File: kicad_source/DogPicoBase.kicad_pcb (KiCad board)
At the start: 2 copper layers, 72 x 53 mm, 52 parts, among them CN1 ARDUINO_ISP, CN2 ARDUINO_MKR, Q1 2N7002, SW1 TAST_VER, SW2 TAST_VER, SW3 TAST_VER, SW4 TAST_VER, SW5 TAST_VER, SW6 TAST_VER, U1 AZ1117IH-3.3, U2 74VHC245D

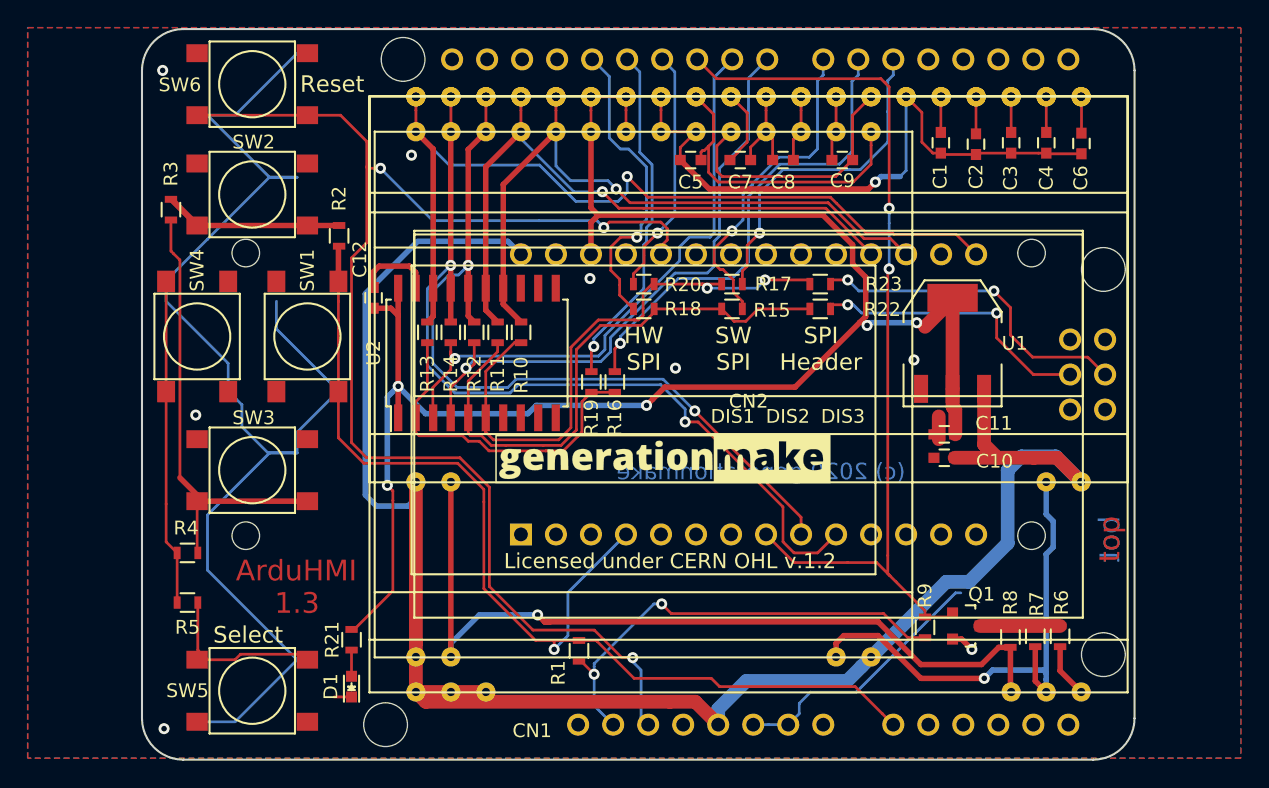
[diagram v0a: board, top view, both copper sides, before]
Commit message: updated schematic
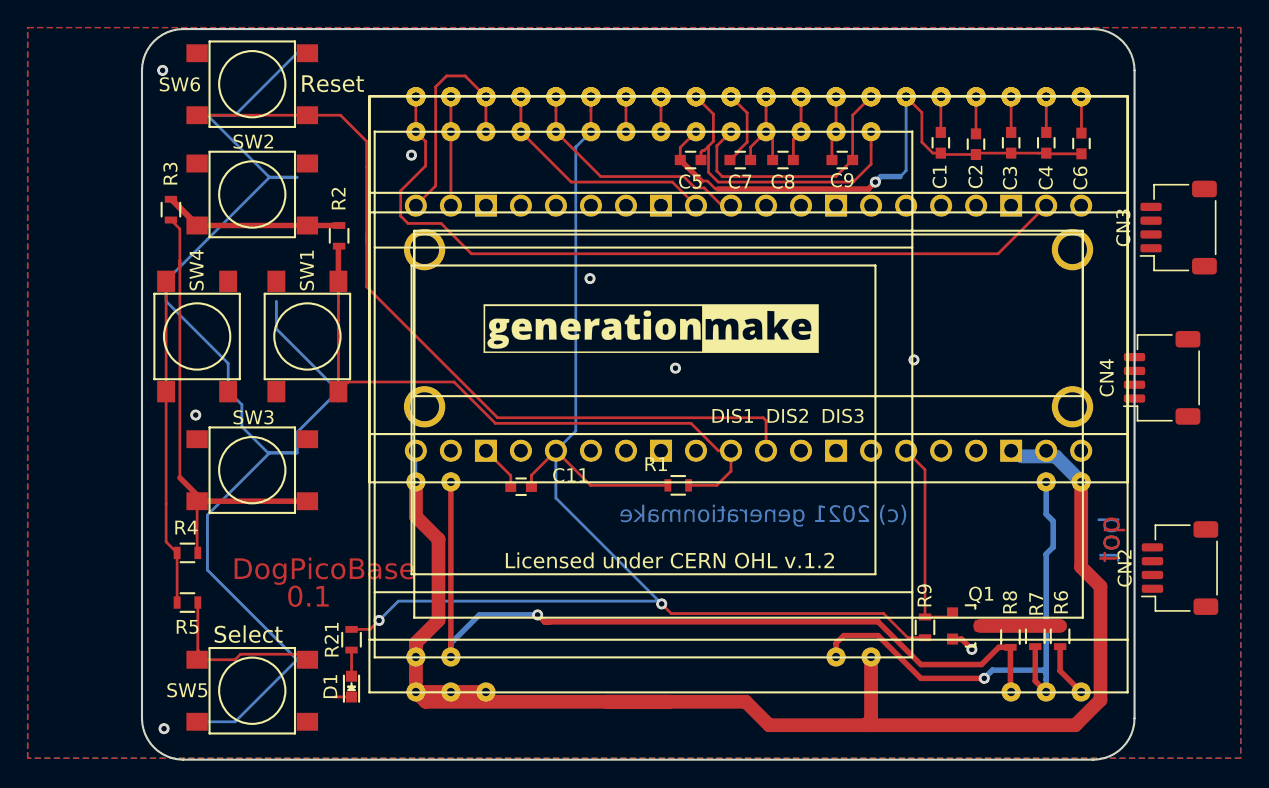
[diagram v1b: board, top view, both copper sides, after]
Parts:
- removed C10: 1uF, capacitors:C_0603
- removed C12: 100nF, capacitors:C_0603
- removed R10, R11, R12, R13, R14, R15, R17, R19, R22, R23: DNI, resistors:R_0603
- removed R16, R18, R20: 0R, resistors:R_0603
- removed U1: AZ1117IH-3.3, SOT_TO:SOT-223
- removed U2: 74VHC245D, SOIC:SOIC-20_7.5x12.8mm_Pitch1.27mm
- added CN3: SM04B-SRSS-TB, Connector_JST:JST_SH_SM04B-SRSS-TB_1x04-1MP_P1.00mm_Horizontal, F.Cu at (126.2, 91.4)
- added CN4: SM04B-SRSS-TB, Connector_JST:JST_SH_SM04B-SRSS-TB_1x04-1MP_P1.00mm_Horizontal, F.Cu at (125.0, 102.3)
- CN1: value ARDUINO_ISP -> RASPBERRYPI_PICO; footprint MODULE_compute:ARDUINO_ISP_TOP -> MODULE_compute:RASPI_PICO; moved to B.Cu
- CN2: value ARDUINO_MKR -> SM04B-SRSS-TB; footprint MODULE_compute:ARDUINO_MKR_HOLES -> Connector_JST:JST_SH_SM04B-SRSS-TB_1x04-1MP_P1.00mm_Horizontal
- moved CN1 51.0 mm to (95.0, 98.7), turned to 270 degrees
- moved CN2 33.7 mm to (126.3, 116.1), turned to 90 degrees
- moved C11 30.9 mm to (78.5, 110.2)
- moved R1 14.0 mm to (89.9, 110.1), turned to 0 degrees
- moved L2 9.49 mm to (87.9, 104.0)
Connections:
- CN1 pad 1: (no net) -> /DIS_A0
- CN1 pad 10: /DISPLAY_BL -> /DIS_SI
- CN1 pad 11: /ARDU_SI_1 -> (no net)
- CN1 pad 12: /ARDU_CS_1 -> (no net)
- CN1 pad 13: /ARDU_CLK_1 -> GND
- CN1 pad 14: GND -> (no net)
- CN1 pad 16: (no net) -> /I2C0_SDA
- CN1 pad 17: (no net) -> /I2C0_SCL
- CN1 pad 18: (no net) -> GND
- CN1 pad 19: (no net) -> /DIS_CS
- CN1 pad 2: (no net) -> /DIS_RESET
- CN1 pad 21: (no net) -> /UART0_TX
- CN1 pad 22: (no net) -> /UART0_RX
- CN1 pad 23: /KEYPAD_A0 -> GND
- CN1 pad 24: (no net) -> /I2C1_SDA
- CN1 pad 25: GND -> /I2C1_SCL
- CN1 pad 26: GND -> /DISPLAY_BL
- CN1 pad 27: +5V -> (no net)
- CN1 pad 28: (no net) -> GND
- CN1 pad 29: /RESET -> (no net)
- CN1 pad 3: (no net) -> GND
- CN1 pad 30: VIO -> /RESET
- CN1 pad 31: (no net) -> /KEYPAD_A0
- CN1 pad 5: /ARDU_SI_2 -> (no net)
- CN1 pad 6: /ARDU_CS_2 -> (no net)
- CN1 pad 7: /ARDU_CLK_2 -> (no net)
- CN1 pad 8: /ARDU_A0 -> GND
- CN1 pad 9: /ARDU_RESET -> /DIS_CLK
- CN2 pad 1: (no net) -> GND
- CN2 pad 2: (no net) -> +3V3
- CN2 pad 3: (no net) -> /UART0_TX
- CN2 pad 4: /KEYPAD_A0 -> /UART0_RX
- R1 pad 1: VIO -> +3V3
- R9 pad 1: VIO -> +3V3
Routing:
- net /DIS_RESET: track 62.7 -> 7.90 mm, vias 2 -> 0
- net /DISPLAY_BL: track 66.7 -> 14.8 mm, vias 2 -> 0
- net /ARDU_A0: track 44.9 -> 0.00 mm, vias 1 -> 0
- net /ARDU_RESET: track 43.5 -> 0.00 mm, vias 1 -> 0
- net /ARDU_SI: track 42.7 -> 0.00 mm, vias 2 -> 0
- net /DIS_A0: track 58.7 -> 16.3 mm, vias 2 -> 0
- net /ARDU_CLK: track 41.0 -> 0.00 mm
- net /RESET: track 97.8 -> 59.4 mm, vias 3 -> 0
- net /ARDU_CS_2: track 34.8 -> 0.00 mm, vias 1 -> 0
- net VIO: track 33.1 -> 0.00 mm, vias 2 -> 0
- net /DIS_SI: track 49.0 -> 17.5 mm, vias 1 -> 0
- net /KEYPAD_A0: track 79.8 -> 48.7 mm, vias 1 -> 0
- net /DIS_CLK: track 47.2 -> 17.5 mm, vias 1 -> 0
- net +3V3: track 128.4 -> 102.2 mm, vias 5 -> 2
- net /ARDU_CS_1: track 25.3 -> 0.00 mm, vias 1 -> 0
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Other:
- board text added: "(c) 2021 generationmake"
- board text added: "0.1"
- board text added: "DogPicoBase"
- board text removed: "(c) 2020 generationmake"
- board text removed: "1.3"
- board text removed: "ArduHMI"
- board text removed: "HW SPI"
- board text removed: "SPI Header"
- board text removed: "SW SPI"
